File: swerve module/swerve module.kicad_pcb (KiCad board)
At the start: 2 copper layers, 63.5 x 37.2 mm, 9 parts, among them J1 MTJ-88ARX1-FSM-LG, J2 MTJ-88ARX1-FSM-LG, J3 CAN out, J4 12v, J5 CAN in, SW1 SW_DPST

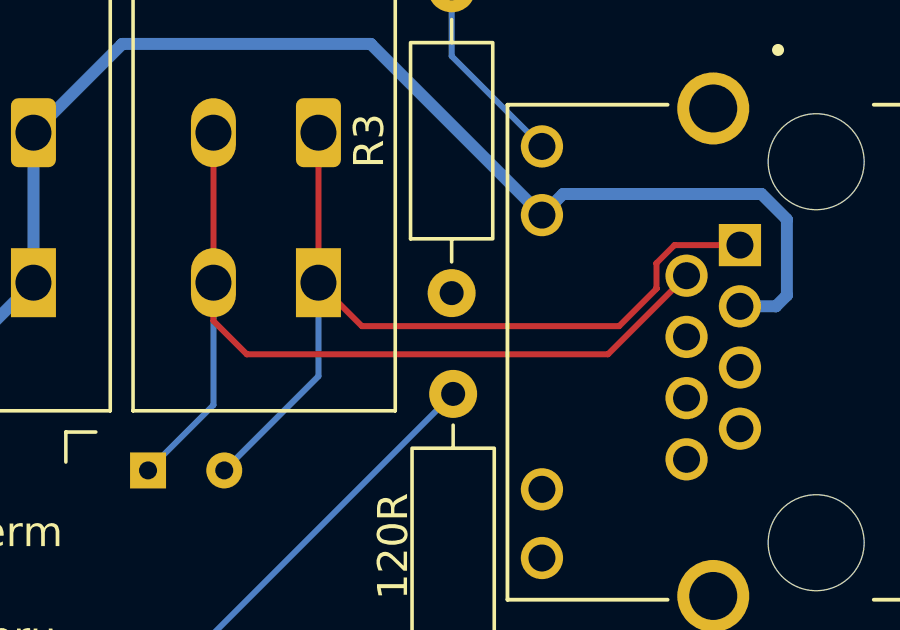
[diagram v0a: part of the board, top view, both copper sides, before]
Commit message: final major changes, exported for JLCPCB
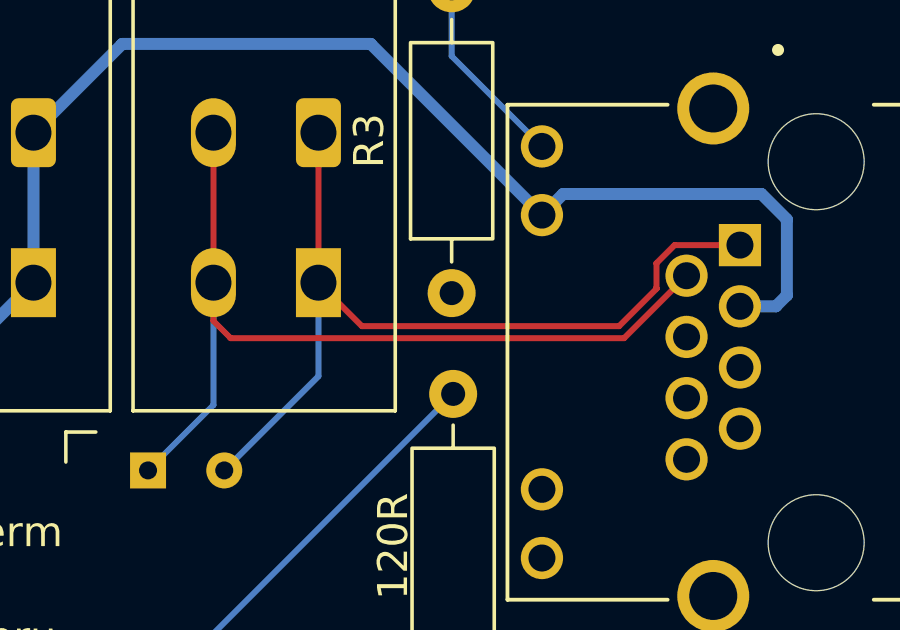
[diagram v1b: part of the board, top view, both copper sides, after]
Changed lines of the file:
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@@
 		(tenting front back)
 		(pcbplotparams
-			(layerselection 0x00000000_00000000_55555555_5755f5ff)
+			(layerselection 0x00000000_00000000_55555555_575555ff)
 			(plot_on_all_layers_selection 0x00000000_00000000_00000000_00000000)
 			(disableapertmacros no)
-			(usegerberextensions no)
-			(usegerberattributes yes)
-			(usegerberadvancedattributes yes)
+			(usegerberextensions yes)
+			(usegerberattributes no)
+			(usegerberadvancedattributes no)
 			(creategerberjobfile yes)
 			(dashed_line_dash_ratio 12.000000)
@@
 			(plotframeref no)
 			(mode 1)
-			(useauxorigin no)
+			(useauxorigin yes)
 			(hpglpennumber 1)
 			(hpglpenspeed 20)
@@
 			(plotpadnumbers no)
 			(hidednponfab no)
-			(sketchdnponfab yes)
-			(crossoutdnponfab yes)
-			(subtractmaskfromsilk no)
+			(sketchdnponfab no)
+			(crossoutdnponfab no)
+			(subtractmaskfromsilk yes)
 			(outputformat 1)
 			(mirror no)
-			(drillshape 1)
+			(drillshape 0)
 			(scaleselection 1)
-			(outputdirectory "")
+			(outputdirectory "JLC/")
 		)
 	)
@@
 	)
 	(segment
-		(start 110.519 56.319)
+		(start 123.098 55.782)
+		(end 109.982 55.782)
+		(width 0.2)
+		(layer "F.Cu")
+		(net 6)
+	)
+	(segment
+		(start 109.982 55.782)
 		(end 109.41 55.21)
 		(width 0.2)
@@
 	)
 	(segment
-		(start 125.18 53.7)
-		(end 122.561 56.319)
-		(width 0.2)
-		(layer "F.Cu")
-		(net 6)
-	)
-	(segment
-		(start 122.561 56.319)
-		(end 110.519 56.319)
-		(width 0.2)
-		(layer "F.Cu")
-		(net 6)
-	)
-	(segment
 		(start 109.41 48.9325)
 		(end 109.41 53.9325)
 		(width 0.2)
 		(layer "F.Cu")
+		(net 6)
+	)
+	(segment
+		(start 125.18 53.7)
+		(end 123.098 55.782)
+		(width 0.2)
+		(layer "F.Cu")
